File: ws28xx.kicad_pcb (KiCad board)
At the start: 4 copper layers, 28.5 x 63.5 mm, 50 parts, among them J1 Conn_02x03_Odd_Even, J2 Conn_02x03_Odd_Even, P1 USB_C_Plug, Q1 S8050, Q2 S8050, Q3 DTC143E, Q4 IRF8736, SW1 io0, SW2 en, U1 TXB0102, U2 ESP32-PICO-D4, U3 FT230XQ, U4 STUSB4500QTR, U5 LM1117-3.3

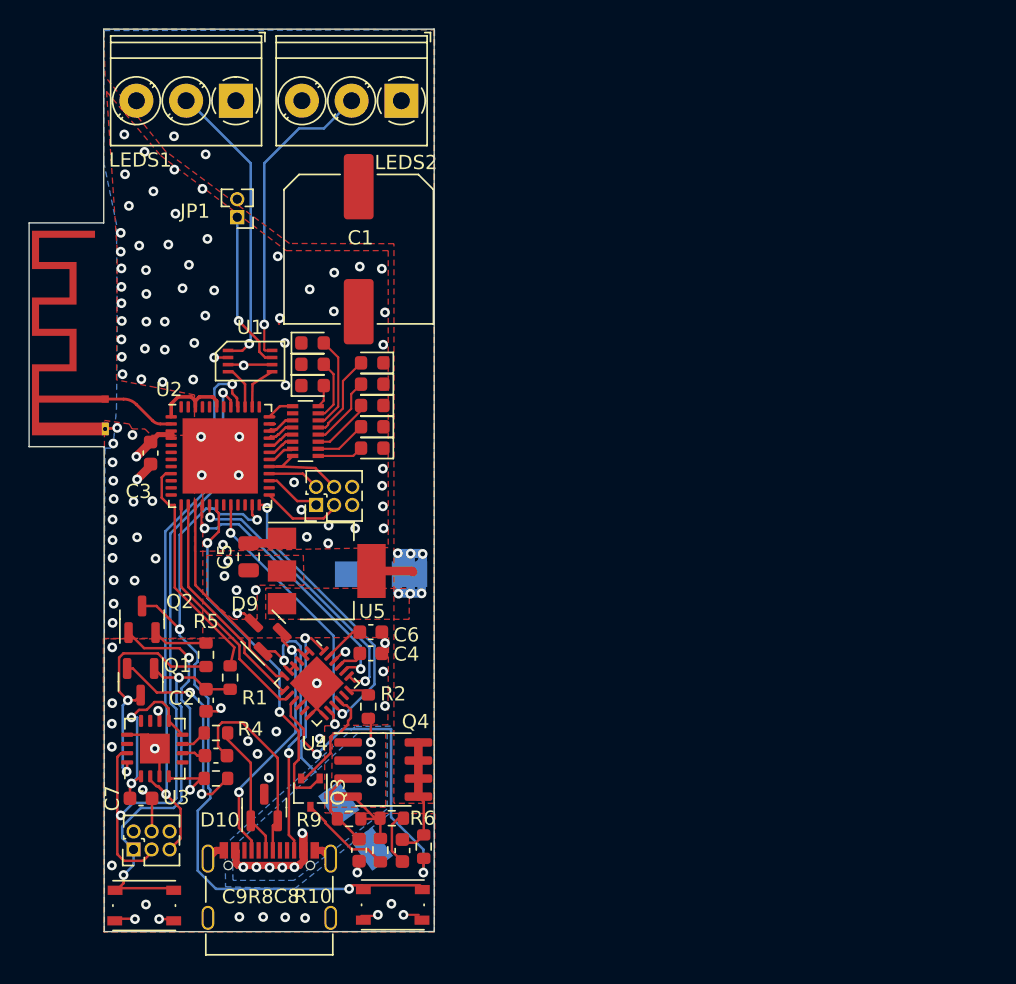
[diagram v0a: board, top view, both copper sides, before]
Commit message: routing
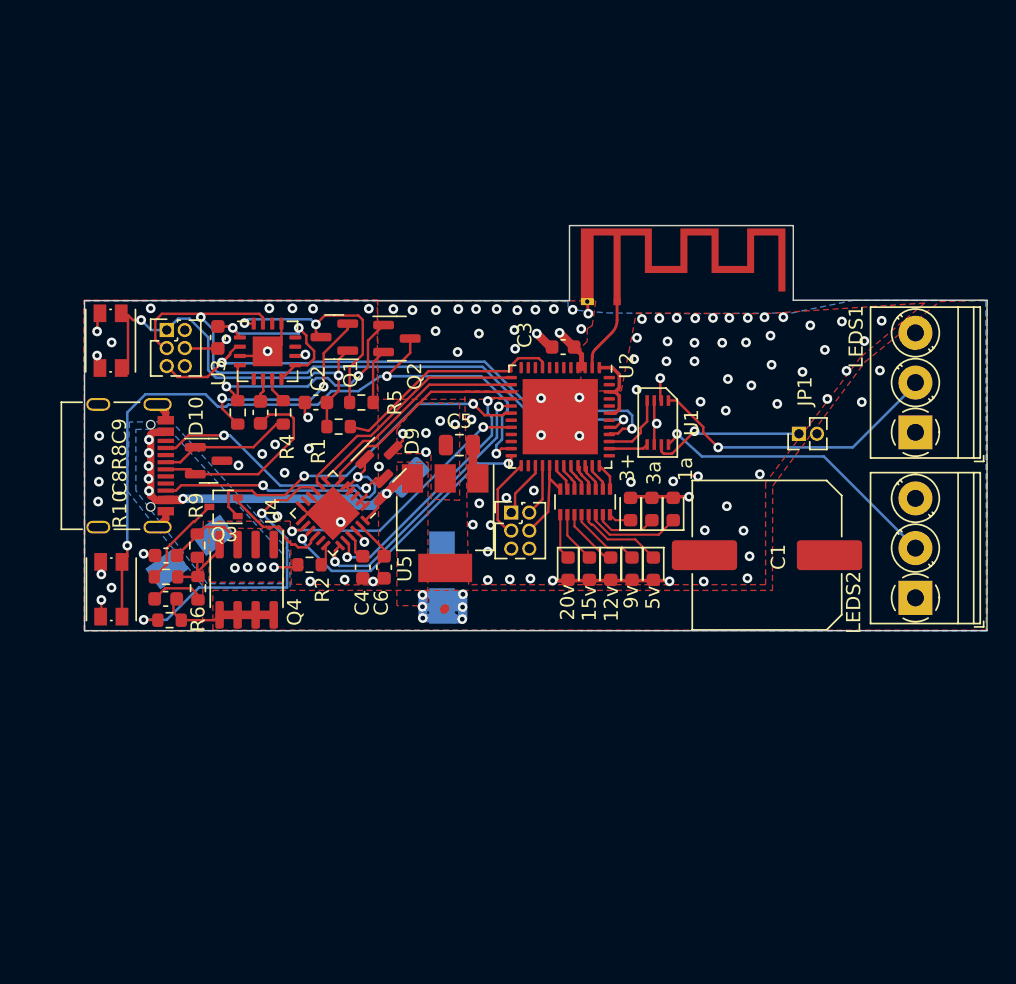
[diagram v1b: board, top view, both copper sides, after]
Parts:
- added C10: 10uf, Capacitor_SMD:C_0805_2012Metric, B.Cu at (134.4, 94.2)
- C1: value C -> 470uf
- SW1, SW2: footprint Button_Switch_SMD:SW_Push_1P1T_NO_Vertical_Wuerth_434133025816 -> precise:SW_Push_1P1T_NO_Vertical
- moved LEDS1 53.2 mm to (170.0, 91.0), turned to 90 degrees
- moved LEDS2 50.3 mm to (170.0, 102.7), turned to 90 degrees
- moved JP1 42.4 mm to (161.8, 91.1), turned to 90 degrees
- moved SW2 39.8 mm to (113.4, 84.6), turned to 90 degrees
- moved AE1 36.7 mm to (149.0, 81.8), turned to 0 degrees
- moved J2 36.6 mm to (117.3, 83.8), turned to 0 degrees
- moved C1 35.9 mm to (159.6, 99.7), turned to 180 degrees
- moved C7 32.9 mm to (120.9, 84.4), turned to -90 degrees
- moved P1 31.2 mm to (114.8, 93.4), turned to -90 degrees
- moved C3 30.0 mm to (145.2, 85.0), turned to 180 degrees
- moved SW1 29.8 mm to (113.4, 102.1), turned to -90 degrees
- moved U3 29.1 mm to (124.4, 85.3), turned to 0 degrees
- moved U1 29.0 mm to (151.9, 90.3), turned to 180 degrees
- moved D4 27.9 mm to (153.0, 96.4), turned to 90 degrees
- moved Q1 27.8 mm to (129.1, 84.3), turned to 180 degrees
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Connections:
- D1 pad 1: GND -> Net-(D1-Pad1)
- D1 pad 2: Net-(D8-Pad2) -> +3V3
- D2 pad 1: GND -> Net-(D2-Pad1)
- D2 pad 2: Net-(D7-Pad2) -> +3V3
- D3 pad 1: GND -> Net-(D3-Pad1)
- D3 pad 2: Net-(D5-Pad2) -> +3V3
- D4 pad 1: GND -> Net-(D4-Pad1)
- D4 pad 2: Net-(D6-Pad2) -> +3V3
- D5 pad 1: GND -> Net-(D5-Pad1)
- D5 pad 2: Net-(D4-Pad2) -> +3V3
- D6 pad 1: GND -> Net-(D6-Pad1)
- D6 pad 2: Net-(D2-Pad2) -> +3V3
- D7 pad 1: GND -> Net-(D7-Pad1)
- D7 pad 2: Net-(D1-Pad2) -> +3V3
- D8 pad 1: GND -> Net-(D8-Pad1)
- D8 pad 2: Net-(D3-Pad2) -> +3V3
- RN1 pad 1: Net-(D1-Pad2) -> Net-(D7-Pad1)
- RN1 pad 10: unconnected-(RN1-Pad10) -> /stat_led6
- RN1 pad 2: Net-(D2-Pad2) -> Net-(D6-Pad1)
- RN1 pad 3: Net-(D3-Pad2) -> Net-(D8-Pad1)
- RN1 pad 4: Net-(D4-Pad2) -> Net-(D5-Pad1)
- RN1 pad 5: Net-(D5-Pad2) -> Net-(D3-Pad1)
- RN1 pad 6: Net-(D6-Pad2) -> Net-(D4-Pad1)
- RN1 pad 7: Net-(D7-Pad2) -> Net-(D2-Pad1)
- RN1 pad 8: Net-(D8-Pad2) -> Net-(D1-Pad1)
- U5 pad 3: VBUS -> VDC
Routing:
- net +3V3: track 8.74 -> 22.3 mm, vias 8 -> 11
- net VDC: track 27.1 -> 36.6 mm
- net Net-(D6-Pad2): track 6.71 -> 0.00 mm
- net Net-(D4-Pad1): track 0.00 -> 6.71 mm
- net Net-(D5-Pad2): track 6.09 -> 0.00 mm
- net Net-(D3-Pad1): track 0.00 -> 6.09 mm
- net Net-(D5-Pad1): track 0.00 -> 5.09 mm
- net Net-(D4-Pad2): track 5.09 -> 0.00 mm
- net Net-(D7-Pad2): track 4.46 -> 0.00 mm
- net Net-(D2-Pad1): track 0.00 -> 4.46 mm
- net Net-(D8-Pad1): track 0.00 -> 3.92 mm
- net Net-(D3-Pad2): track 3.92 -> 0.00 mm
- net Net-(D6-Pad1): track 0.00 -> 3.65 mm
- net Net-(D2-Pad2): track 3.65 -> 0.00 mm
- net Net-(D7-Pad1): track 0.00 -> 3.24 mm
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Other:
- board size 28.5 x 63.5 mm -> 63.5 x 28.5 mm
- board text added: "12v"
- board text added: "15v"
- board text added: "1a"
- board text added: "20v"
- board text added: "3+"
- board text added: "3a"
- board text added: "5v"
- board text added: "9v"
